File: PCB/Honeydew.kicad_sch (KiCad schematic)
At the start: 6 parts, among them J9 RGB_EX

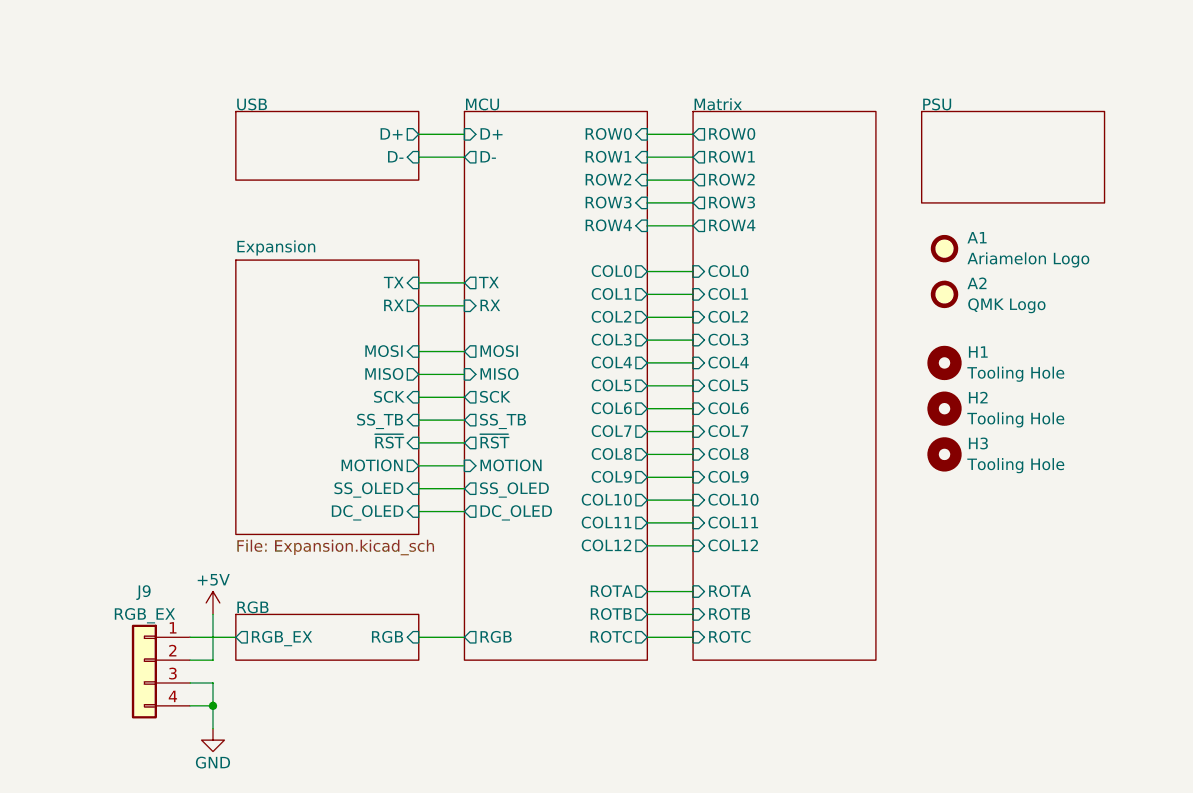
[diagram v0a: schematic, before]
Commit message: Large update.
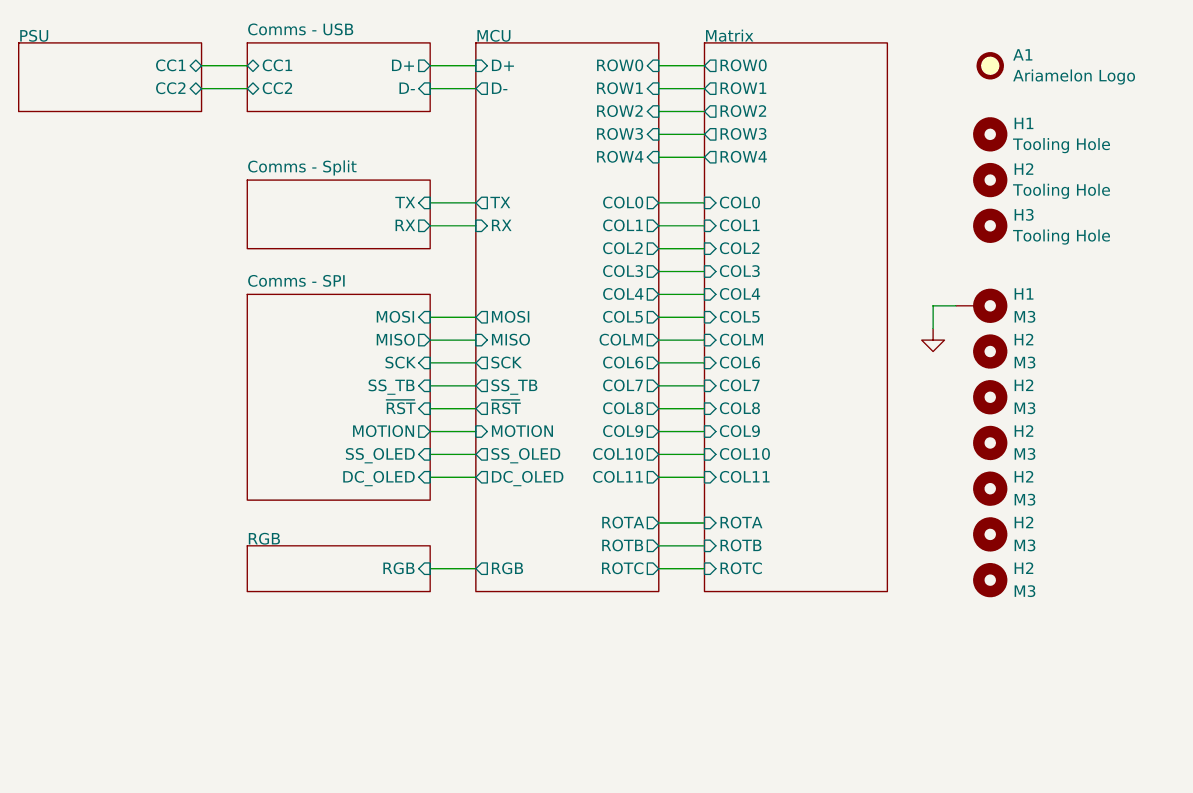
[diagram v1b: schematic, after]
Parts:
- removed A2: QMK Logo, Honeydew:QMK Logo, symbol Mechanical:Fiducial
- removed J9: RGB_EX, Honeydew:PinHeader_1x04_P2.54mm_Vertical_SIlkless, symbol Connector_Generic:Conn_01x04
- added H1: M3, Honeydew:MountingHole_3.2mm_M3_Pad, symbol Mechanical:MountingHole_Pad
- added H2 (x6): M3, Honeydew:MountingHole_3.2mm_M3_Pad, symbol Mechanical:MountingHole
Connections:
- net GND: now also H1.1
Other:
- removed sheet Expansion
- removed sheet USB
- added sheet Comms - SPI (Comms-SPI.kicad_sch)
- added sheet Comms - Split (Comms - Split.kicad_sch)
- added sheet Comms - USB (Comms-USB.kicad_sch)
- sheet MCU ports: added COLM; removed COL12
- sheet Matrix ports: added COLM; removed COL12
- sheet PSU ports: added CC1, CC2; removed none
- sheet RGB ports: added none; removed RGB_EX
- moved on the sheet: A1, H1, H2, H3
